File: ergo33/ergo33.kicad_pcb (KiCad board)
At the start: 2 copper layers, 173.8 x 121.8 mm, 135 parts, among them M1 MountingHole_2.2mm_M2_ISO7380, M2 MountingHole_2.2mm_M2_ISO7380, SW1 SW_Push, SW46 Rotary_Encoder_Switch, U1 ATmega32U4-AU, U2 USBLC6-2SC6, Y1 16MHz

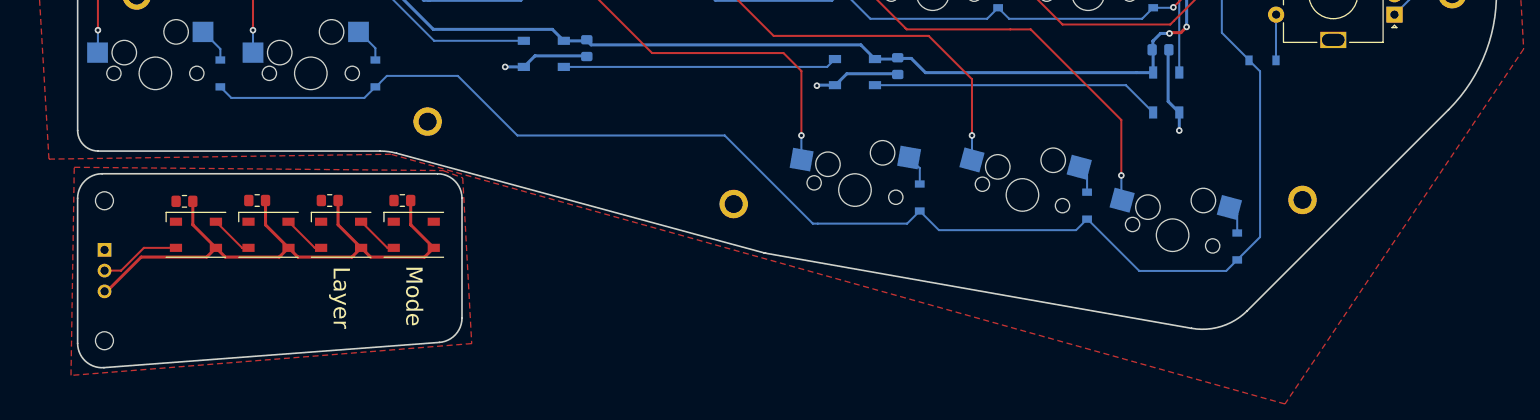
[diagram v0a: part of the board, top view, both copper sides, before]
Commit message: ergo33: minor tweaking
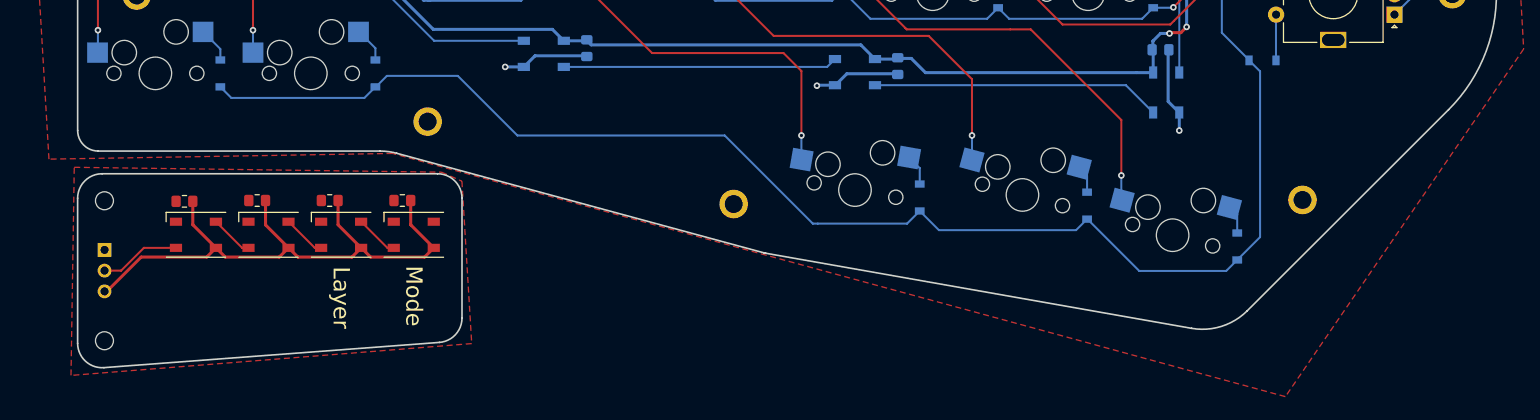
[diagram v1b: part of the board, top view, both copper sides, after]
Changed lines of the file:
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@@
     (polygon
       (pts
-        (xy 196.8 27.4) (xy 201 101.5) (xy 171.75 145) (xy 62.2 114.4) (xy 20.3 115)
+        (xy 196.8 27.4) (xy 201 101.5) (xy 171.8 144.1) (xy 62.4 114.3) (xy 20.3 115)
         (xy 14.7 20) (xy 23.2 16.5) (xy 82.2 16.5)
       )
@@
     (polygon
       (pts
-        (xy 68.6 116.4) (xy 71 117.3) (xy 72.1 137.6) (xy 23 141.5) (xy 23.4 116)
+        (xy 68.4 116.6) (xy 70.9 117.7) (xy 72.1 137.6) (xy 23 141.5) (xy 23.4 116)
       )
     )
